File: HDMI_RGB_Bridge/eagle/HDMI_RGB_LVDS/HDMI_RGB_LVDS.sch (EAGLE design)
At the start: 95 parts, among them CON1 KLDX-0202-A-LT, CON2 FCI-10029449-111RLF, CON3 XF2M-4015-1A, CON4 FCI-10033526-N3212LF, CON5 MOLEX-53261-0671, CON6 FI-X30SSLA-HF, IC1 WPMDL1300501BD, IC2 WPMDL1300331BD, IC3 TLV1117CDCYR, IC4 AT24C01C-SSHM-B, IC5 TFP401APZP, IC6 ATMEGA48A-AU, IC7 FT232RL, IC8 SN75LVDS83BDGGR, Q1 ATS073ASM-1, T1 IRF9530NSTRRPBF, T2 IRLML2502TRPBF

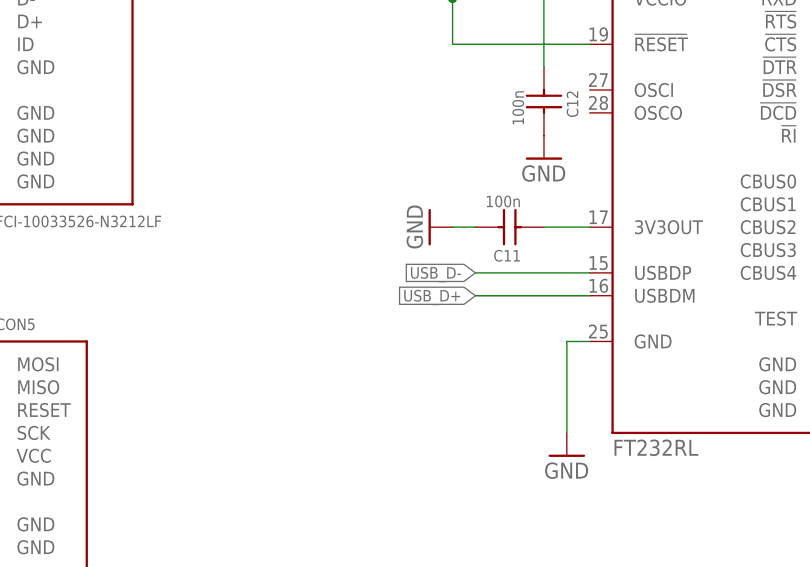
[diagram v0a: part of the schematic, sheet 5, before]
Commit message: end of workday 24.03.2014
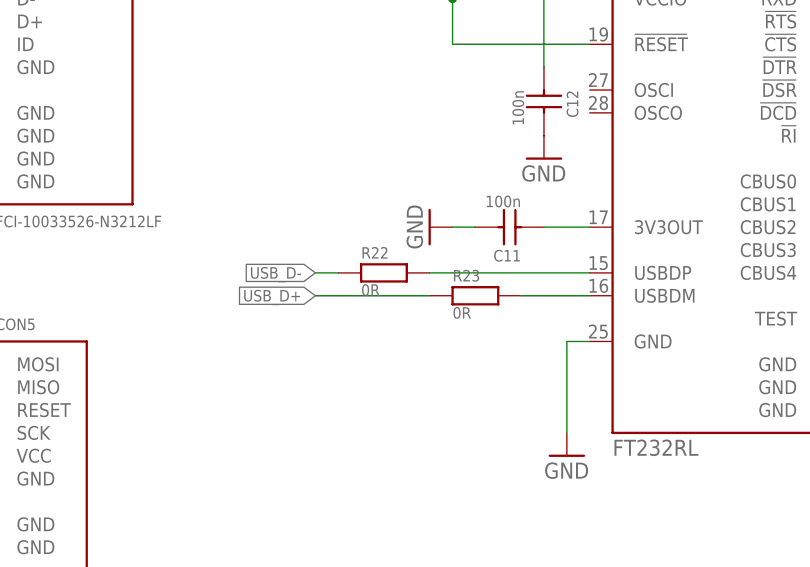
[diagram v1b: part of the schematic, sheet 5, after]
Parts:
- added R22, R23: 0R, SchlegelAr_Master:R0402
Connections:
- new net N$10: IC7.USBDM, R23.P$2
- new net N$5: IC7.USBDP, R22.P$2
- net USB_D+: now also R23.P$1; no longer IC7.USBDM
- net USB_D-: now also R22.P$1; no longer IC7.USBDP
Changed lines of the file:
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@@
 <part name="SP18" library="SchlegelAr_Master" deviceset="SP2" device=""/>
 <part name="U$35" library="SchlegelAr_Master" deviceset="+5V" device=""/>
+<part name="R22" library="SchlegelAr_Master" deviceset="R" device="0402" value="0R"/>
+<part name="R23" library="SchlegelAr_Master" deviceset="R" device="0402" value="0R"/>
 </parts>
 <sheets>
@@
 <instance part="SP13" gate="G$1" x="152.4" y="182.88"/>
 <instance part="U$35" gate="G$1" x="142.24" y="195.58"/>
+<instance part="R22" gate="G$1" x="76.2" y="200.66"/>
+<instance part="R23" gate="G$1" x="86.36" y="198.12"/>
 </instances>
 <busses>
@@
 </segment>
 <segment>
-<wire x1="99.06" y1="200.66" x2="86.36" y2="200.66" width="0.1524" layer="91"/>
-<label x="86.36" y="200.66" size="1.27" layer="95" rot="R180" xref="yes"/>
-<pinref part="IC7" gate="G$1" pin="USBDP"/>
+<label x="68.58" y="200.66" size="1.27" layer="95" rot="R180" xref="yes"/>
+<wire x1="71.12" y1="200.66" x2="68.58" y2="200.66" width="0.1524" layer="91"/>
+<pinref part="R22" gate="G$1" pin="P$1"/>
 </segment>
 </net>
@@
 </segment>
 <segment>
-<wire x1="99.06" y1="198.12" x2="86.36" y2="198.12" width="0.1524" layer="91"/>
-<label x="86.36" y="198.12" size="1.27" layer="95" rot="R180" xref="yes"/>
-<pinref part="IC7" gate="G$1" pin="USBDM"/>
+<label x="68.58" y="198.12" size="1.27" layer="95" rot="R180" xref="yes"/>
+<wire x1="81.28" y1="198.12" x2="68.58" y2="198.12" width="0.1524" layer="91"/>
+<pinref part="R23" gate="G$1" pin="P$1"/>
 </segment>
 </net>
@@
 </segment>
 </net>
+<net name="N$5" class="0">
+<segment>
+<pinref part="R22" gate="G$1" pin="P$2"/>
+<pinref part="IC7" gate="G$1" pin="USBDP"/>
+<wire x1="81.28" y1="200.66" x2="99.06" y2="200.66" width="0.1524" layer="91"/>
+</segment>
+</net>
+<net name="N$10" class="0">
+<segment>
+<pinref part="IC7" gate="G$1" pin="USBDM"/>
+<pinref part="R23" gate="G$1" pin="P$2"/>
+<wire x1="99.06" y1="198.12" x2="91.44" y2="198.12" width="0.1524" layer="91"/>
+</segment>
+</net>
